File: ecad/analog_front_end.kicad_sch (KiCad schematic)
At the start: 44 parts, among them J1 DUT, J2 Switch, J4 Switch, J6 Switch, J7 Switch, U1 LM6144xIx, U2 LM4030-4.096, U4 ADS8328IPW

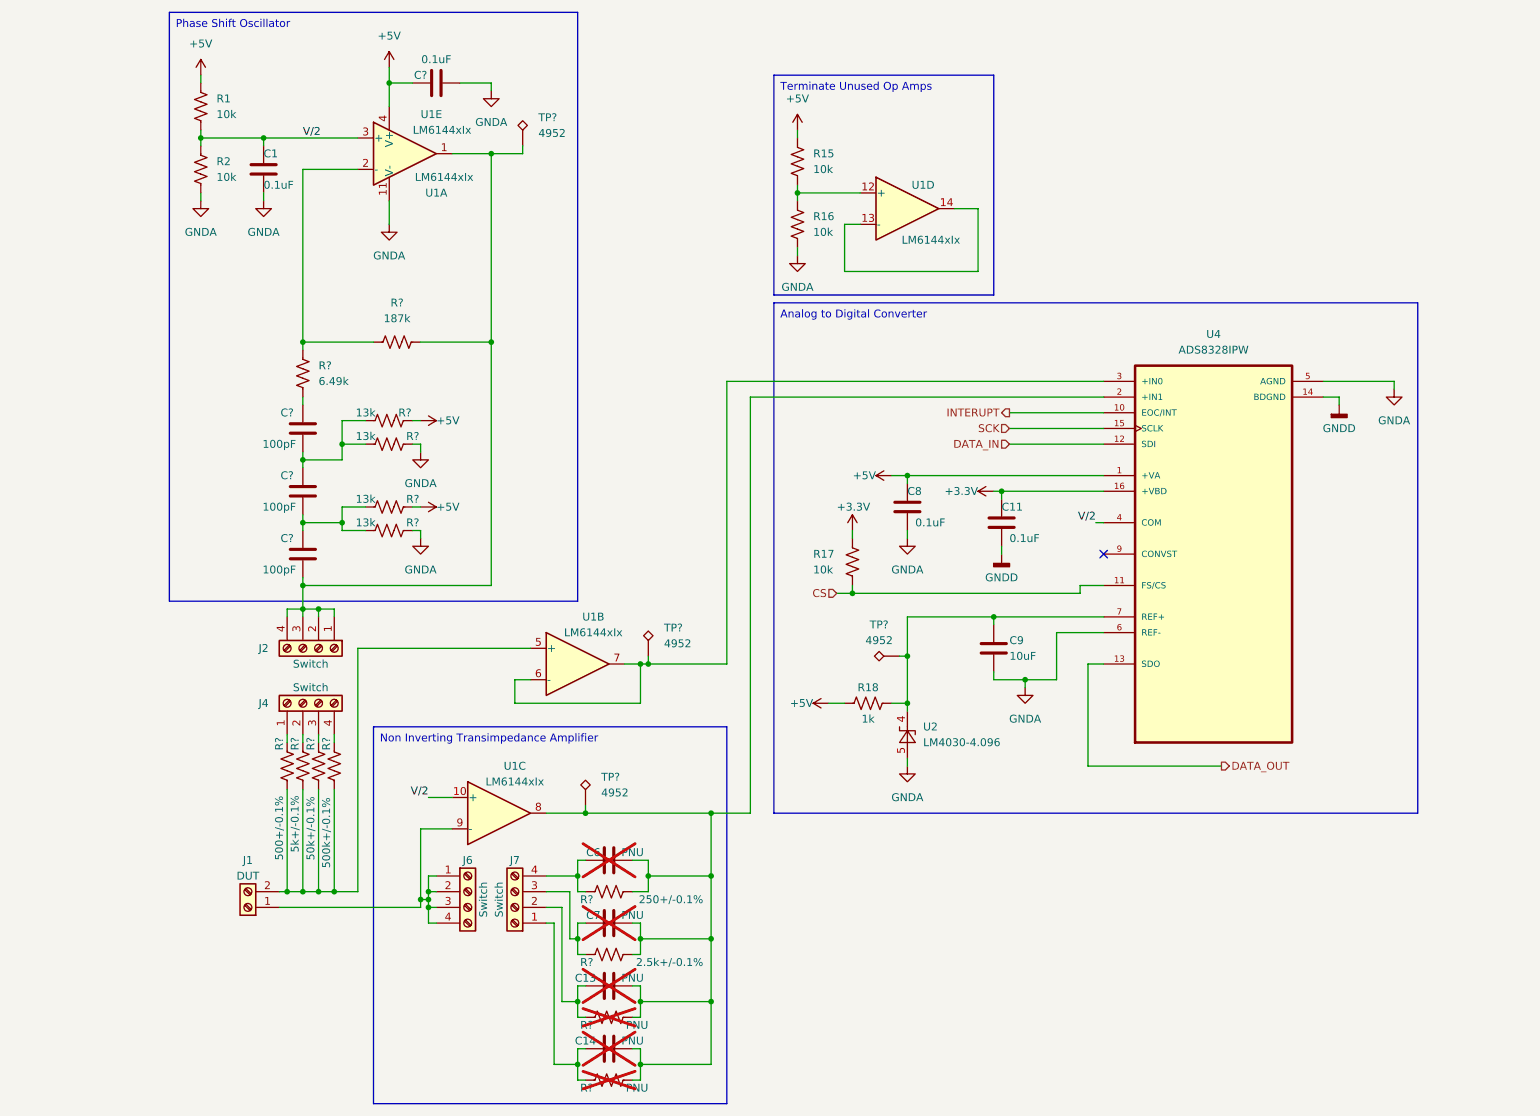
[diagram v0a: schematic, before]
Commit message: layout draft
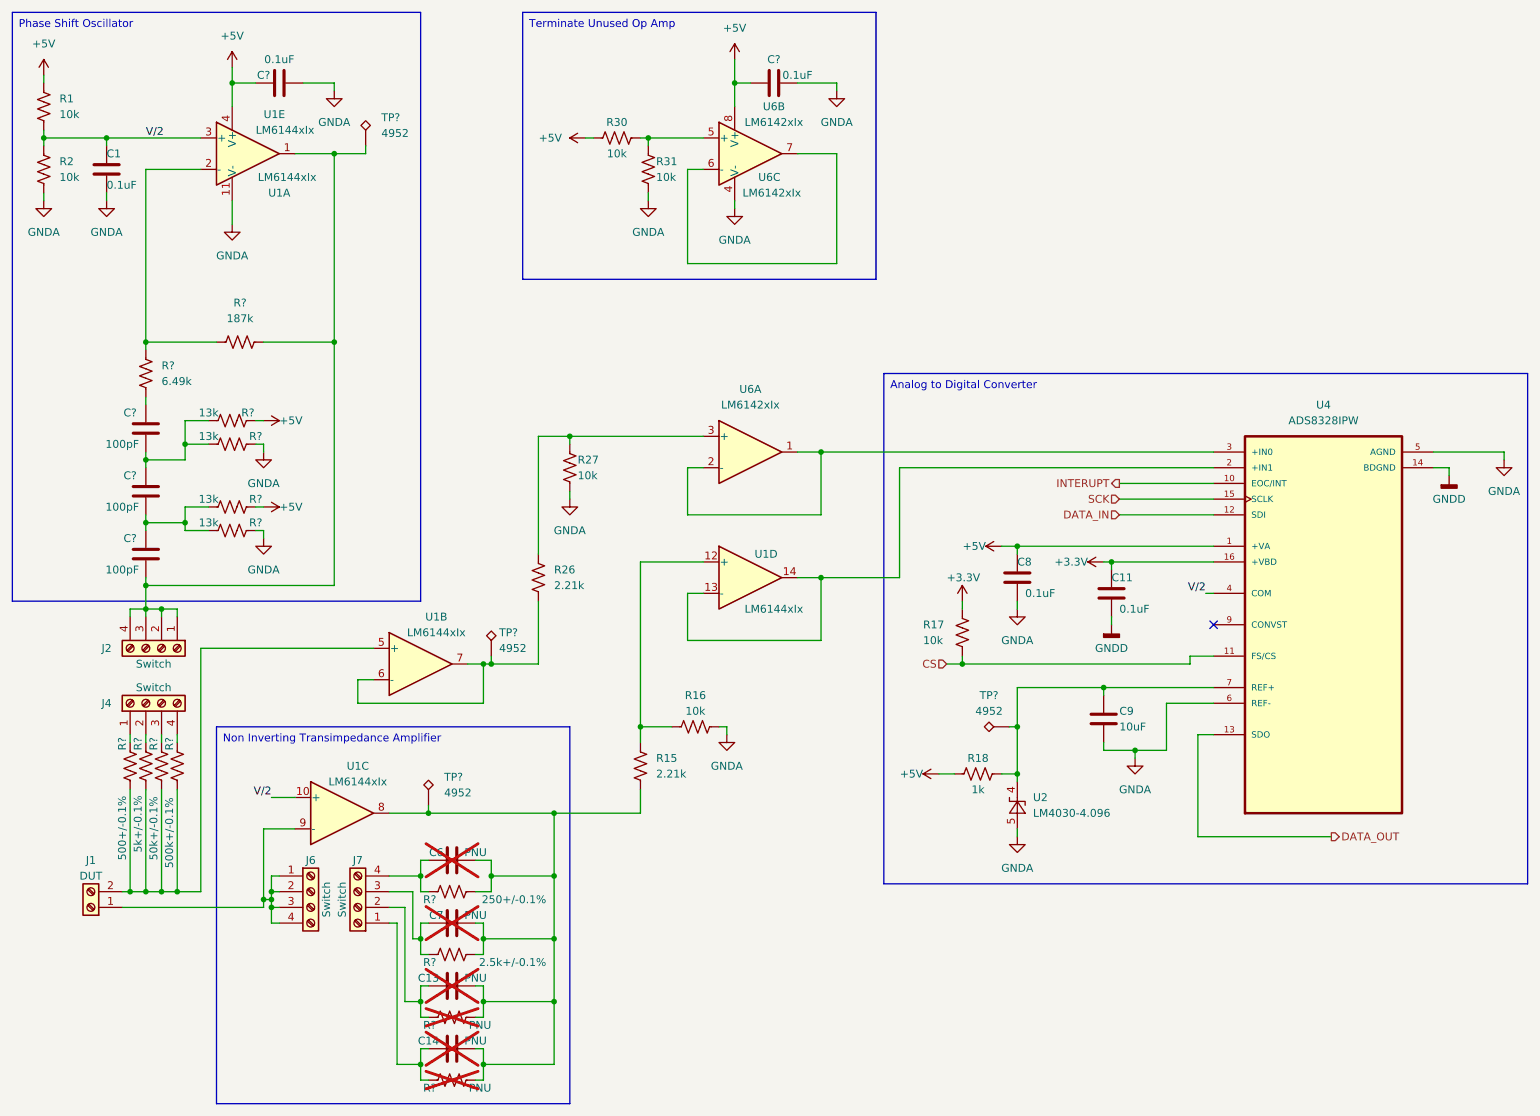
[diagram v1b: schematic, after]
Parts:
- added C?: 0.1uF, Capacitor_SMD:C_0805_2012Metric, symbol Device:C
- added R26: 2.21k, Resistor_SMD:R_0805_2012Metric, symbol Device:R_US
- added R27, R30, R31: 10k, Resistor_SMD:R_0805_2012Metric, symbol Device:R_US
- added U6: LM6142xIx, Package_DIP:DIP-8_W7.62mm, symbol Amplifier_Operational:LM6142xIx
- R15: value 10k -> 2.21k
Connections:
- net +5V: now also C?.1, R30.1, U6.8 (V+); no longer R15.1
- net GNDA: now also C?.2, R27.2, R31.1, U6.4 (V-)
- net at C13.2, C14.2, C6.2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: now also R15.2; no longer U4.2 (+IN1)
- net at R16.1, U1.12 (+): now also R15.1; no longer R15.2
- net at TP?.1, U1.6 (-), U1.7: now also R26.2; no longer U4.3 (+IN0)
- net at U1.13 (-), U1.14: now also U4.2 (+IN1)
- new net: R30.2, R31.2, U6.5 (+)
- new net: U6.6 (-), U6.7
- new net: U4.3 (+IN0), U6.1, U6.2 (-)
- new net: R26.1, R27.1, U6.3 (+)
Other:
- title: Inductance and Capacitance Meter Analog Front End -> LCR Meter Analog Front End
- moved on the sheet: C1, C11, C13, C14, C6, C7, C8, C9, C?, J1, J2, J4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
